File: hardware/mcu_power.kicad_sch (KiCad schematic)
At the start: 85 parts, among them Q201 MMBT3904, Q202 IRLML2244, SW201 Button Power, SW202 Reset, SW203 Button Enter, SW204 Button Left, SW205 Button Up, SW206 Button Down, SW207 Button Escape, SW208 Button Right, U201 STM32F405RGTx, U202 TPS7A2033, U203 TP6841S6, Y201 8 MHz

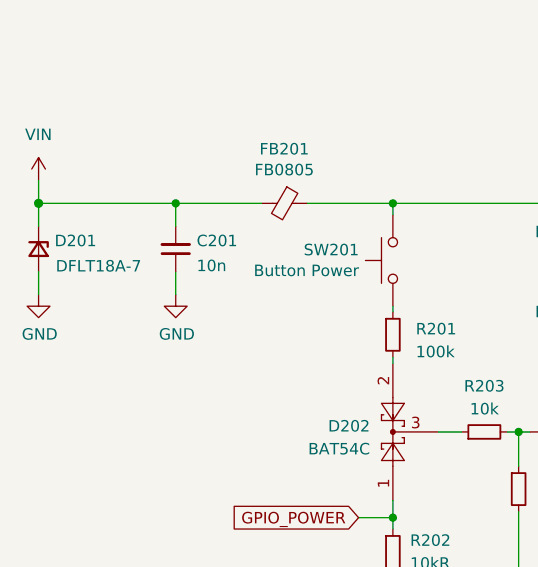
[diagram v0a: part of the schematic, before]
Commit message: PCB Layout [WIP]
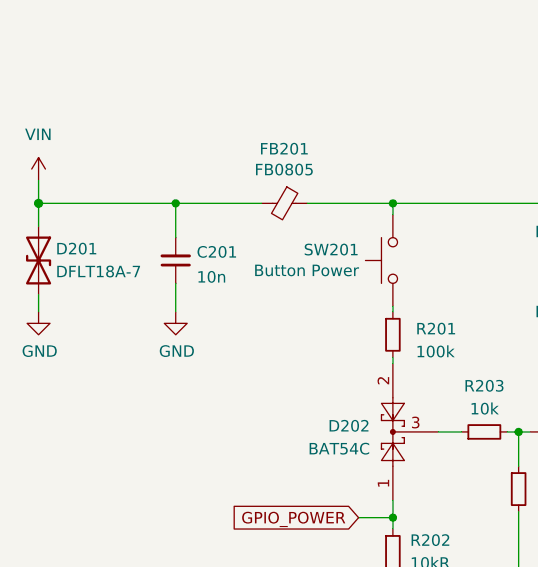
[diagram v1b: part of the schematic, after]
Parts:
- removed D201: DFLT18A-7, Diode_SMD:D_SOD-128, symbol Device:D_Zener_Small
- added D201: DFLT18A-7, Diode_SMD:D_SOD-128, symbol Device:D_TVS
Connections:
- net GND: now also D201.2 (A2)
- net VIN: now also D201.1 (A1)
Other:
- moved on the sheet: C201
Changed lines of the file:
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@@
     (stroke (width 0) (type default))
   )
-  (wire (pts (xy 34.925 153.67) (xy 34.925 156.21))
+  (wire (pts (xy 34.925 154.94) (xy 34.925 158.115))
     (stroke (width 0) (type solid))
   )
@@
     (stroke (width 0) (type solid))
   )
+  (wire (pts (xy 19.685 156.21) (xy 19.685 158.115))
+    (stroke (width 0) (type default))
+  )
   (wire (pts (xy 259.08 118.745) (xy 256.54 118.745))
     (stroke (width 0) (type solid))
@@
     (stroke (width 0) (type solid))
   )
-  (wire (pts (xy 19.685 153.67) (xy 19.685 156.21))
-    (stroke (width 0) (type solid))
-  )
   (wire (pts (xy 93.98 24.13) (xy 93.98 21.59))
     (stroke (width 0) (type solid))
@@
     (stroke (width 0) (type solid))
   )
-  (wire (pts (xy 34.925 146.05) (xy 34.925 148.59))
+  (wire (pts (xy 34.925 146.05) (xy 34.925 149.86))
     (stroke (width 0) (type solid))
   )
@@
     )
   )
-  (symbol (lib_id "power:GND") (at 19.685 156.21 0) (unit 1)
+  (symbol (lib_id "power:GND") (at 19.685 158.115 0) (unit 1)
     (in_bom yes) (on_board yes) (dnp no)
-    (property "Reference" "#PWR0202" (at 19.685 162.56 0)
+    (property "Reference" "#PWR0202" (at 19.685 164.465 0)
       (effects (font (size 1.27 1.27)) hide)
     )
-    (property "Value" "GND" (at 19.812 160.6042 0)
+    (property "Value" "GND" (at 19.812 162.5092 0)
       (effects (font (size 1.27 1.27)))
     )
-    (property "Footprint" "" (at 19.685 156.21 0)
+    (property "Footprint" "" (at 19.685 158.115 0)
       (effects (font (size 1.27 1.27)) hide)
     )
-    (property "Datasheet" "" (at 19.685 156.21 0)
+    (property "Datasheet" "" (at 19.685 158.115 0)
       (effects (font (size 1.27 1.27)) hide)
     )
@@
     )
   )
+  (symbol (lib_id "Device:D_TVS") (at 19.685 152.4 270) (unit 1)
+    (in_bom yes) (on_board yes) (dnp no)
+    (property "Reference" "D201" (at 21.59 151.13 90)
+      (effects (font (size 1.27 1.27)) (justify left))
+    )
+    (property "Value" "DFLT18A-7 " (at 21.59 153.67 90)
+      (effects (font (size 1.27 1.27)) (justify left))
+    )
+    (property "Footprint" "Diode_SMD:D_SOD-128" (at 19.685 152.4 0)
+      (effects (font (size 1.27 1.27)) hide)
+    )
+    (property "Datasheet" "~" (at 19.685 152.4 0)
+      (effects (font (size 1.27 1.27)) hide)
+    )
+    (property "LCSC Part #" "C2909295" (at 19.685 152.4 0)
+      (effects (font (size 1.27 1.27)) hide)
+    )
+    (property "MPN" "DFLT18A-7" (at 19.685 152.4 0)
+      (effects (font (size 1.27 1.27)) hide)
+    )
+    (pin "1")
+    (pin "2")
+    (instances
+      (project "M17-SmartMic"
+        (path "/59592280-3207-432b-a891-cd517ec5cf12/00000000-0000-0000-0000-0000612c95ef"
+          (reference "D201") (unit 1)
+        )
+      )
+    )
+  )
   (symbol (lib_id "power:+5V") (at 249.555 144.78 0) (unit 1)
     (in_bom yes) (on_board yes) (dnp no) (fields_autoplaced)
@@
     )
   )
-  (symbol (lib_id "Device:D_Zener_Small") (at 19.685 151.13 270) (unit 1)
-    (in_bom no) (on_board yes) (dnp no)
-    (property "Reference" "D201" (at 21.4631 150.2215 90)
-      (effects (font (size 1.27 1.27)) (justify left))
-    )
-    (property "Value" "DFLT18A-7 " (at 21.59 153.035 90)
-      (effects (font (size 1.27 1.27)) (justify left))
-    )
-    (property "Footprint" "Diode_SMD:D_SOD-128" (at 19.685 151.13 90)
-      (effects (font (size 1.27 1.27)) hide)
-    )
-    (property "Datasheet" "~" (at 19.685 151.13 90)
-      (effects (font (size 1.27 1.27)) hide)
-    )
-    (property "MPN" "DFLT18A-7" (at 19.685 151.13 0)
-      (effects (font (size 1.27 1.27)) hide)
-    )
-    (property "LCSC Part #" "C2909295" (at 19.685 151.13 0)
-      (effects (font (size 1.27 1.27)) hide)
-    )
-    (pin "1")
-    (pin "2")
-    (instances
-      (project "M17-SmartMic"
-        (path "/59592280-3207-432b-a891-cd517ec5cf12/00000000-0000-0000-0000-0000612c95ef"
-          (reference "D201") (unit 1)
-        )
-      )
-    )
-  )
   (symbol (lib_id "pkl_power:VIN") (at 19.685 143.51 0) (unit 1)
     (in_bom yes) (on_board yes) (dnp no) (fields_autoplaced)
@@
     )
   )
-  (symbol (lib_id "pkl_device:pkl_C_Small") (at 34.925 151.13 180) (unit 1)
+  (symbol (lib_id "pkl_device:pkl_C_Small") (at 34.925 152.4 180) (unit 1)
     (in_bom yes) (on_board yes) (dnp no) (fields_autoplaced)
-    (property "Reference" "C201" (at 37.2492 150.2215 0)
+    (property "Reference" "C201" (at 37.2492 151.4915 0)
       (effects (font (size 1.27 1.27)) (justify right))
     )
-    (property "Value" "10n" (at 37.2492 152.9966 0)
+    (property "Value" "10n" (at 37.2492 154.2666 0)
       (effects (font (size 1.27 1.27)) (justify right))
     )
-    (property "Footprint" "pkl_dipol:C_0603" (at 34.925 151.13 0)
+    (property "Footprint" "pkl_dipol:C_0603" (at 34.925 152.4 0)
       (effects (font (size 1.524 1.524)) hide)
     )
-    (property "Datasheet" "" (at 34.925 151.13 0)
+    (property "Datasheet" "" (at 34.925 152.4 0)
       (effects (font (size 1.524 1.524)))
     )
-    (property "MPN" "Generic C/10nF/C0G/25V/0603" (at 34.925 151.13 0)
+    (property "MPN" "Generic C/10nF/C0G/25V/0603" (at 34.925 152.4 0)
       (effects (font (size 1.27 1.27)) hide)
     )
@@
     )
   )
-  (symbol (lib_id "power:GND") (at 34.925 156.21 0) (unit 1)
+  (symbol (lib_id "power:GND") (at 34.925 158.115 0) (unit 1)
     (in_bom yes) (on_board yes) (dnp no)
-    (property "Reference" "#PWR0204" (at 34.925 162.56 0)
+    (property "Reference" "#PWR0204" (at 34.925 164.465 0)
       (effects (font (size 1.27 1.27)) hide)
     )
-    (property "Value" "GND" (at 35.052 160.6042 0)
+    (property "Value" "GND" (at 35.052 162.5092 0)
       (effects (font (size 1.27 1.27)))
     )
-    (property "Footprint" "" (at 34.925 156.21 0)
+    (property "Footprint" "" (at 34.925 158.115 0)
       (effects (font (size 1.27 1.27)) hide)
     )
-    (property "Datasheet" "" (at 34.925 156.21 0)
+    (property "Datasheet" "" (at 34.925 158.115 0)
       (effects (font (size 1.27 1.27)) hide)
     )
